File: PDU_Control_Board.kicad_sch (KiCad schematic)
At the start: 237 parts

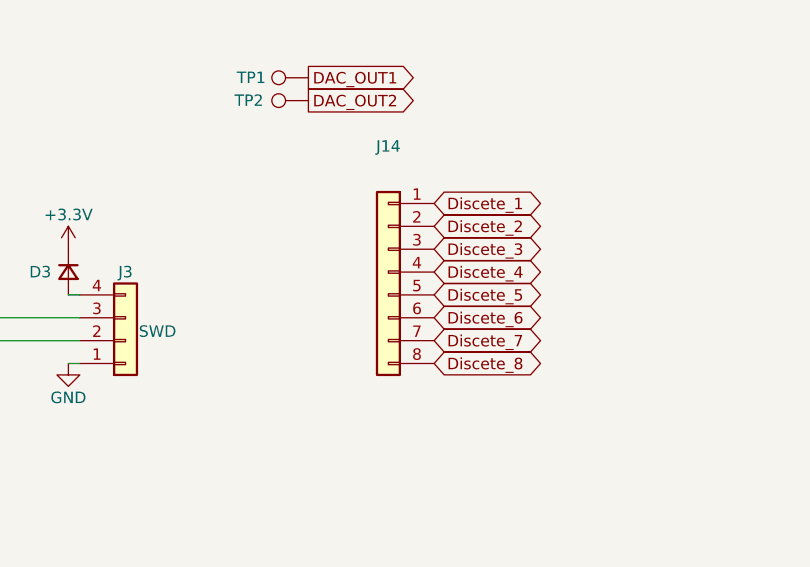
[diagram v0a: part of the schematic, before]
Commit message: VER3.0: заказал плату в резоните
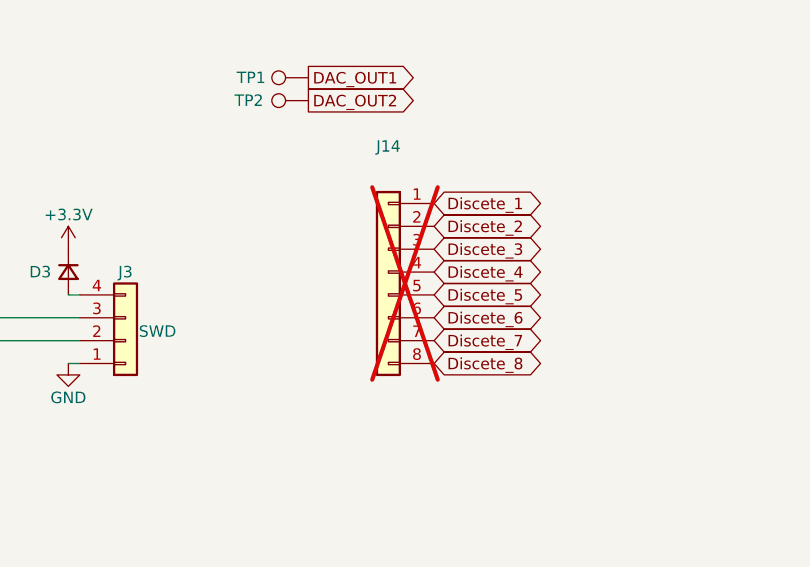
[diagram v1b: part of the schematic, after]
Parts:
- J14: now not fitted
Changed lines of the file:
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@@
 		(in_bom yes)
 		(on_board yes)
-		(dnp no)
+		(dnp yes)
 		(fields_autoplaced yes)
 		(property "Reference" "J14"
